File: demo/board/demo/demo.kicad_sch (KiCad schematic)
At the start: 21 parts, among them J6 Conn_01x05, U1 STM32F413CGUx, U2 LD1117S33TR_SOT223, U4 MCP2551-I-SN, Y1 CSTNE8M00

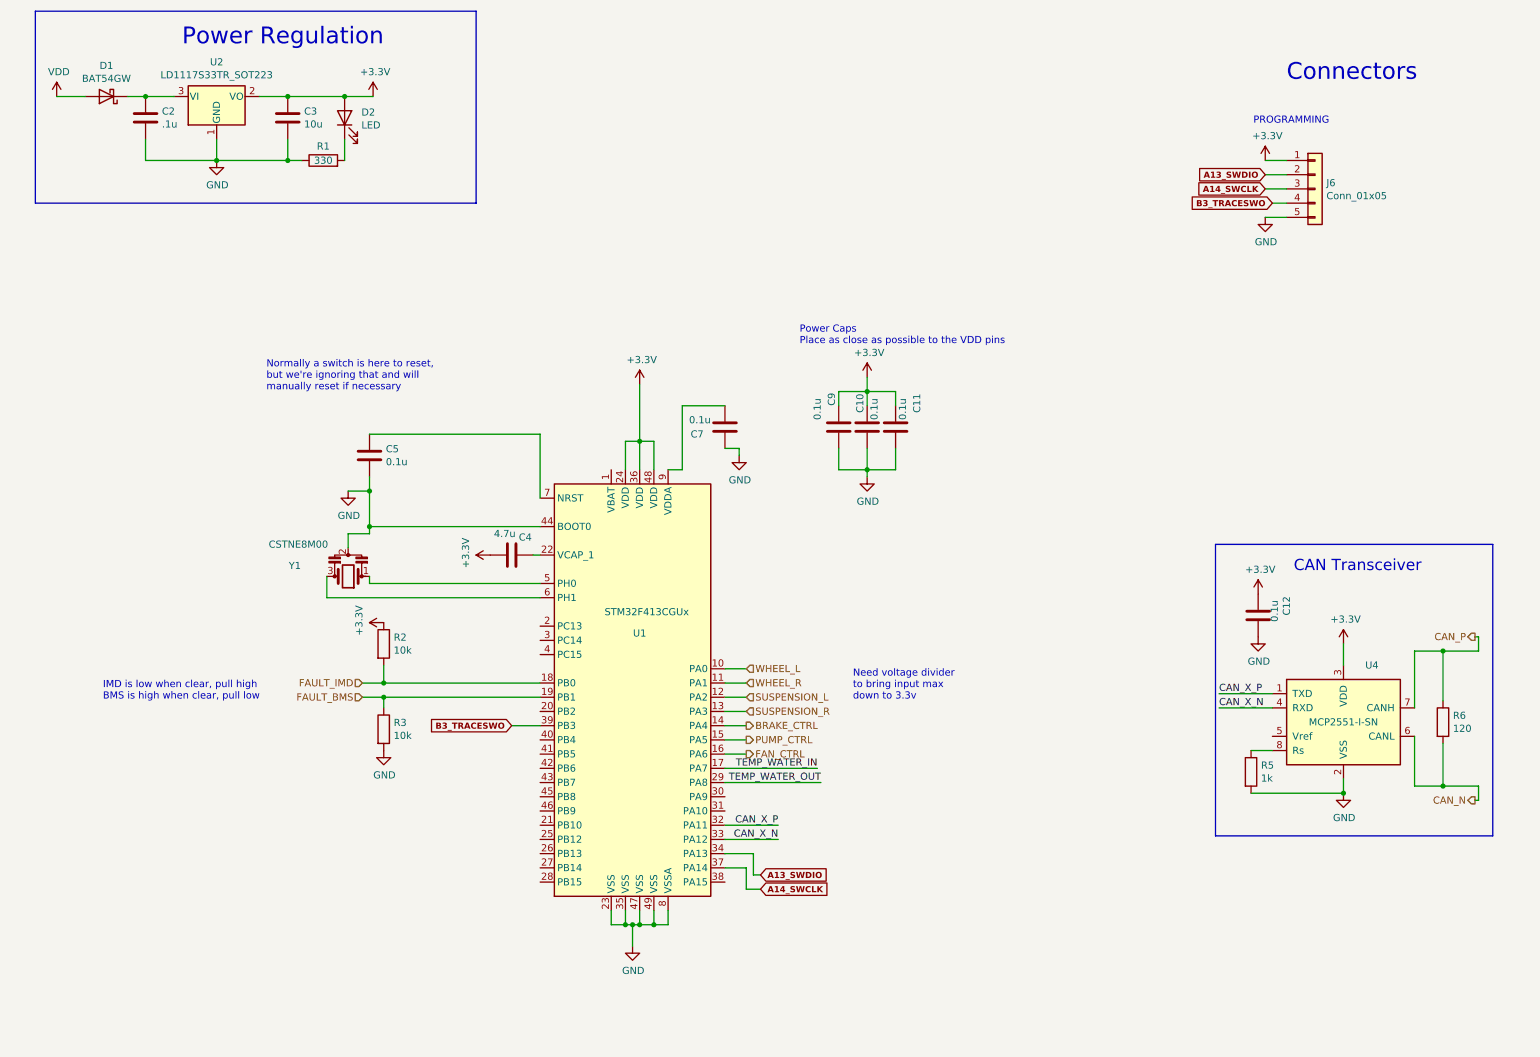
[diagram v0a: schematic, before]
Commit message: updating demo schem
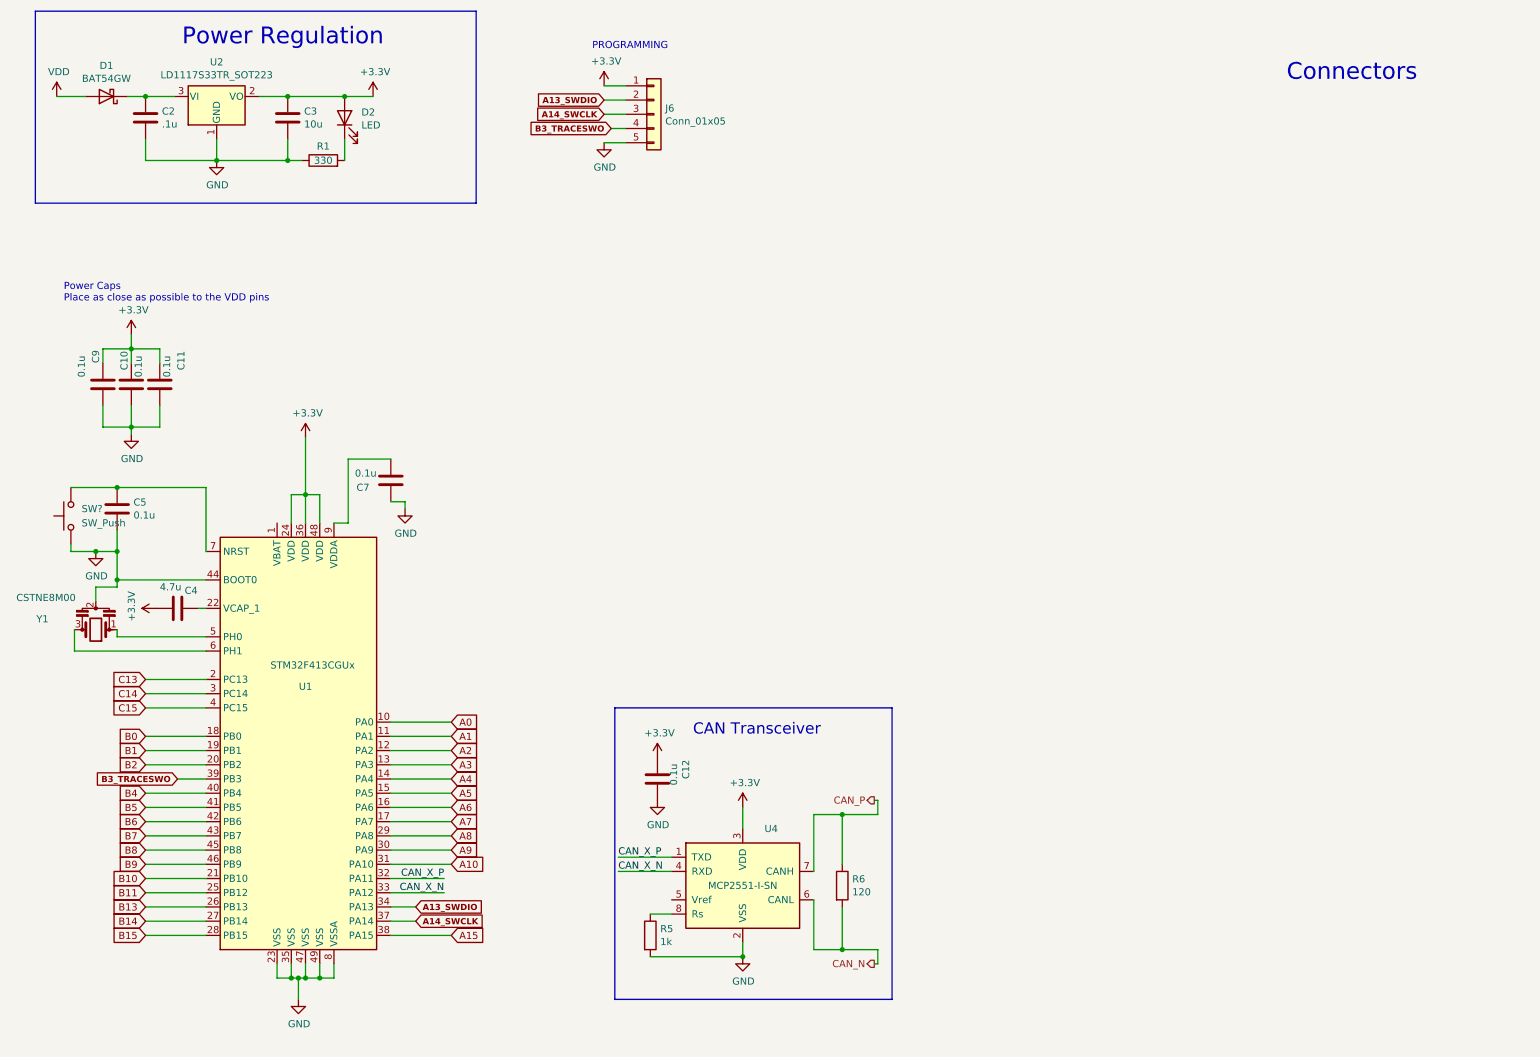
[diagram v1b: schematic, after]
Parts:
- removed R2, R3: 10k, Resistor_SMD:R_0603_1608Metric_Pad0.98x0.95mm_HandSolder, symbol Device:R
- added SW?: SW_Push, symbol Switch:SW_Push
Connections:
- net GND: now also SW?.1
- net C13: now reaches U1.2 (PC13)
- net B2: now reaches U1.20 (PB2)
- net B10: now reaches U1.21 (PB10)
- net B11: now reaches U1.25 (PB12)
- net B13: now reaches U1.26 (PB13)
- net B14: now reaches U1.27 (PB14)
- net B15: now reaches U1.28 (PB15)
- net C14: now reaches U1.3 (PC14)
- net A9: now reaches U1.30 (PA9)
- net A10: now reaches U1.31 (PA10)
- net A15: now reaches U1.38 (PA15)
- net C15: now reaches U1.4 (PC15)
- net B4: now reaches U1.40 (PB4)
- net B5: now reaches U1.41 (PB5)
- net B6: now reaches U1.42 (PB6)
- net B7: now reaches U1.43 (PB7)
- net B8: now reaches U1.45 (PB8)
- net B9: now reaches U1.46 (PB9)
- net at C5.1, U1.7 (NRST): now also SW?.2
- net BRAKE_CTRL renamed A4
- net FAN_CTRL renamed A6
- net FAULT_BMS renamed B1
- net FAULT_IMD renamed B0
- net PUMP_CTRL renamed A5
- net SUSPENSION_L renamed A2
- net SUSPENSION_R renamed A3
- net TEMP_WATER_IN renamed A7
- net TEMP_WATER_OUT renamed A8
- net WHEEL_L renamed A0
- net WHEEL_R renamed A1
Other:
- note removed: "IMD is low when clear, pull high BMS is high when clear, pull low"
- note removed: "Need voltage divider to bring input max down to 3.3v"
- note removed: "Normally a switch is here to reset, but we're ignoring that and will manually reset if necessary"
- moved on the sheet: C10, C11, C12, C4, C5, C7, C9, J6, R5, R6, U1, U4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

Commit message: working on demo board, schem done
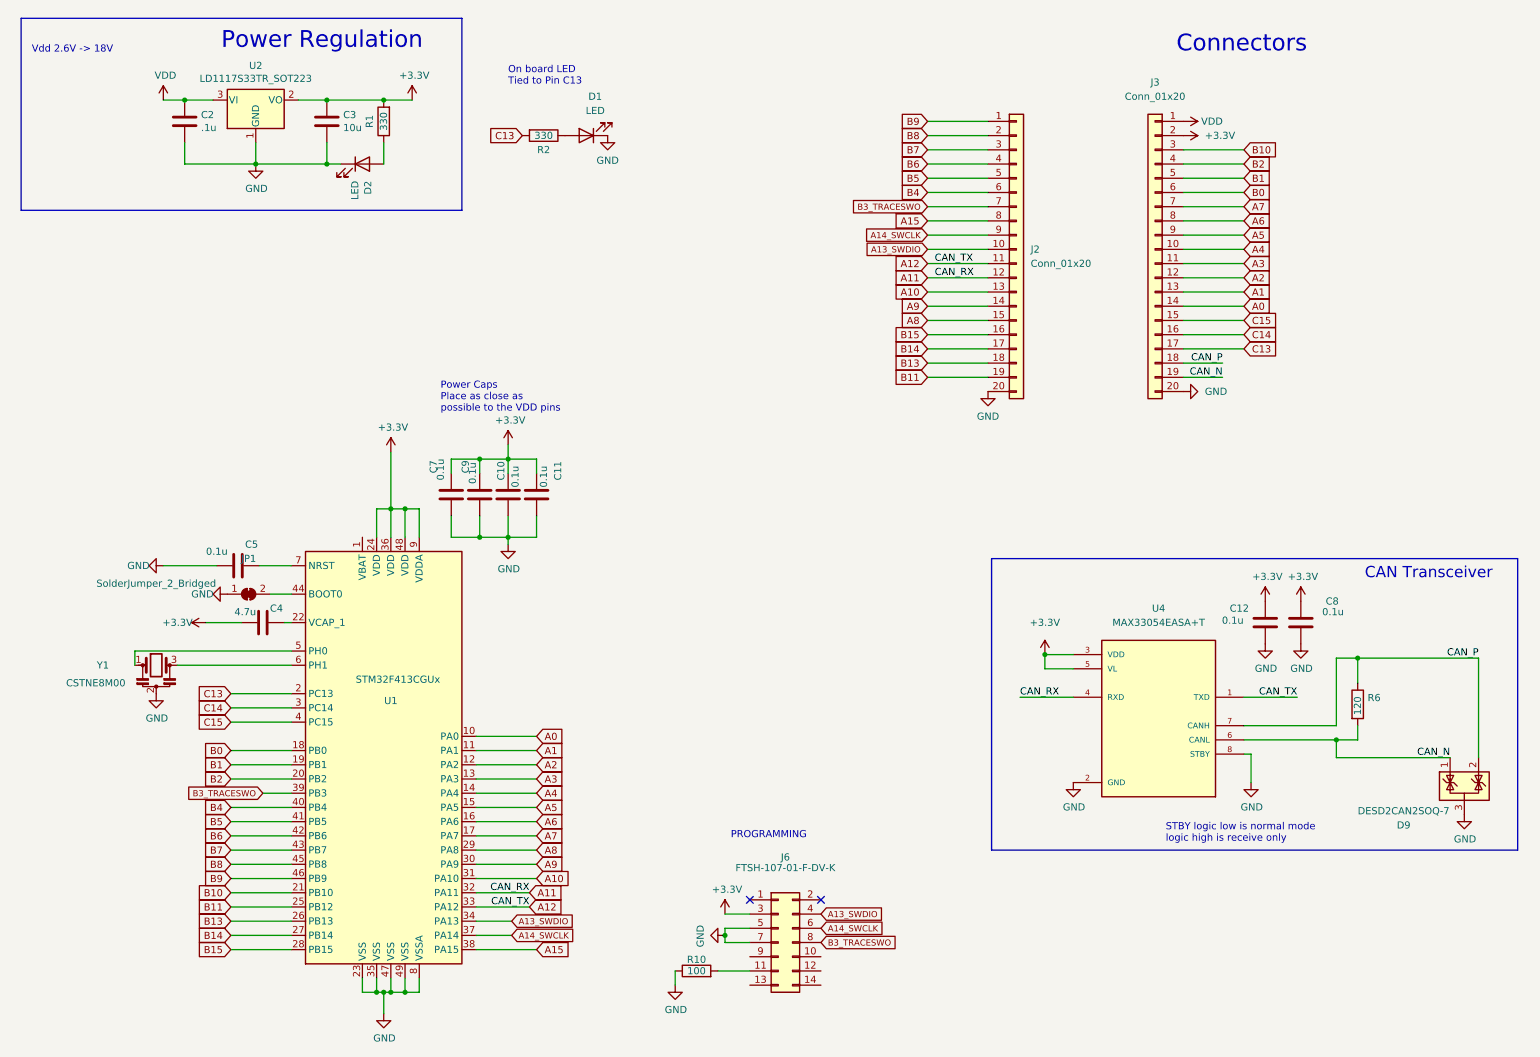
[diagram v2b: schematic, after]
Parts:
- removed D1: BAT54GW, Diode_SMD:D_SMB, symbol Device:D_Schottky
- removed J6: Conn_01x05, Connector_JST:JST_XH_B5B-XH-A_1x05_P2.50mm_Vertical, symbol Connector_Generic:Conn_01x05
- removed R5: 1k, Resistor_SMD:R_0603_1608Metric_Pad0.98x0.95mm_HandSolder, symbol Device:R
- removed SW?: SW_Push, symbol Switch:SW_Push
- removed U4: MCP2551-I-SN, Package_SO:SOIC-8_3.9x4.9mm_P1.27mm, symbol Interface_CAN_LIN:MCP2551-I-SN
- added C8: 0.1u, Capacitor_SMD:C_0603_1608Metric_Pad1.08x0.95mm_HandSolder, symbol Device:C
- added D1: LED, LED_SMD:LED_0603_1608Metric_Pad1.05x0.95mm_HandSolder, symbol Device:LED
- added D9: DESD2CAN2SOQ-7, Package_TO_SOT_SMD:SOT-23, symbol Power_Protection:NUP2105L
- added J2, J3: Conn_01x20, Connector_PinHeader_2.54mm:PinHeader_1x20_P2.54mm_Vertical, symbol Connector_Generic:Conn_01x20
- added J6: FTSH-107-01-F-DV-K, Connector_PinHeader_1.27mm:PinHeader_2x07_P1.27mm_Vertical_SMD, symbol Connector_Generic:Conn_02x07_Odd_Even
- added JP1: SolderJumper_2_Bridged, Jumper:SolderJumper-2_P1.3mm_Bridged_RoundedPad1.0x1.5mm, symbol Jumper:SolderJumper_2_Bridged
- added R10: 100, Resistor_SMD:R_0603_1608Metric_Pad0.98x0.95mm_HandSolder, symbol Device:R
- added R2: 330, Resistor_SMD:R_0603_1608Metric_Pad0.98x0.95mm_HandSolder, symbol Device:R
- added U4: MAX33054EASA+T, AERO_Footprints:SOIC127P600X175-8N, symbol AERO_Symbols:MAX33054EASA+T
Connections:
- net +3V3: now also C7.1, R1.2, U1.9 (VDDA), C8.1, J3.2 (Pin_2), J6.3 (Pin_3), U4.3 (VDD), U4.5 (VL); no longer D2.2 (A)
- net A0: now also J3.14 (Pin_14)
- net A1: now also J3.13 (Pin_13)
- net A10: now also J2.13 (Pin_13)
- net A13_SWDIO: now also J2.10 (Pin_10), J6.4 (Pin_4)
- net A14_SWCLK: now also J2.9 (Pin_9), J6.6 (Pin_6)
- net A15: now also J2.8 (Pin_8)
- net A2: now also J3.12 (Pin_12)
- net A3: now also J3.11 (Pin_11)
- net A4: now also J3.10 (Pin_10)
- net A5: now also J3.9 (Pin_9)
- net A6: now also J3.8 (Pin_8)
- net A7: now also J3.7 (Pin_7)
- net A8: now also J2.15 (Pin_15)
- net A9: now also J2.14 (Pin_14)
- net B0: now also J3.6 (Pin_6)
- net B1: now also J3.5 (Pin_5)
- net B10: now also J3.3 (Pin_3)
- net B11: now also J2.19 (Pin_19)
- net B13: now also J2.18 (Pin_18)
- net B14: now also J2.17 (Pin_17)
- net B15: now also J2.16 (Pin_16)
- net B2: now also J3.4 (Pin_4)
- net B3_TRACESWO: now also J2.7 (Pin_7), J6.8 (Pin_8)
- net B4: now also J2.6 (Pin_6)
- net B5: now also J2.5 (Pin_5)
- net B6: now also J2.4 (Pin_4)
- net B7: now also J2.3 (Pin_3)
- net B8: now also J2.2 (Pin_2)
- net B9: now also J2.1 (Pin_1)
- net C13: now also J3.17 (Pin_17), R2.2
- net C14: now also J3.16 (Pin_16)
- net C15: now also J3.15 (Pin_15)
- net CAN_N: now also D9.1 (K), J3.19 (Pin_19), U4.6 (CANL)
- net CAN_P: now also D9.2 (K), J3.18 (Pin_18), U4.7 (CANH)
- net GND: now also C7.2, D2.1 (K), C8.2, D1.1 (K), D9.3 (A), J2.20 (Pin_20), J3.20 (Pin_20), J6.5 (Pin_5), J6.7 (Pin_7), JP1.1 (A), R10.1, U4.2 (GND), U4.8 (STBY); no longer C7.1, R1.1, U1.44 (BOOT0)
- net VDD: now also C2.1, U2.3 (VI), J3.1 (Pin_1)
- net CAN_X_N renamed A12
- net A12: now also J2.11 (Pin_11), U4.1 (TXD)
- net CAN_X_P renamed A11
- net A11: now also J2.12 (Pin_12), U4.4 (RXD)
- new net: D2.2 (A), R1.1
- new net: JP1.2 (B), U1.44 (BOOT0)
- new net: J6.11 (Pin_11), R10.2
- new net: D1.2 (A), R2.1
- no-connect marks 0 -> 2
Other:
- note added: "On board LED Tied to Pin C13"
- note added: "STBY logic low is normal mode logic high is receive only"
- note added: "Vdd 2.6V -> 18V"
- moved on the sheet: C2, C3, D2, R1, U2
